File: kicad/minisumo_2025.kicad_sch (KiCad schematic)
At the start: 5 parts

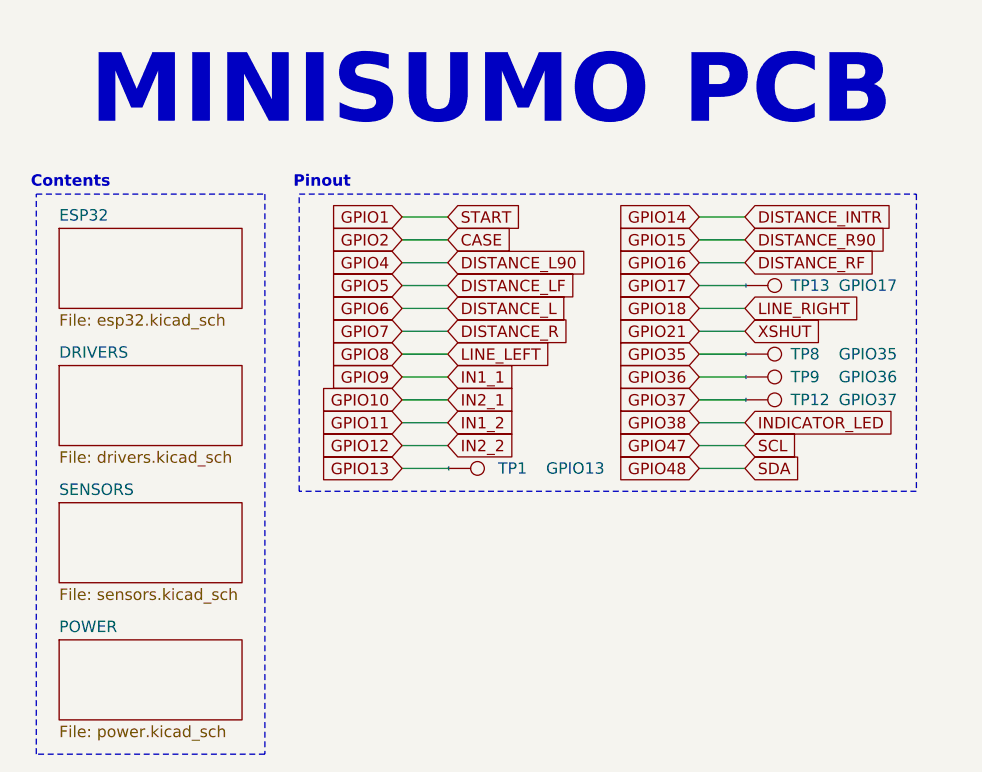
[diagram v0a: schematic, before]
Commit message: 2026 version
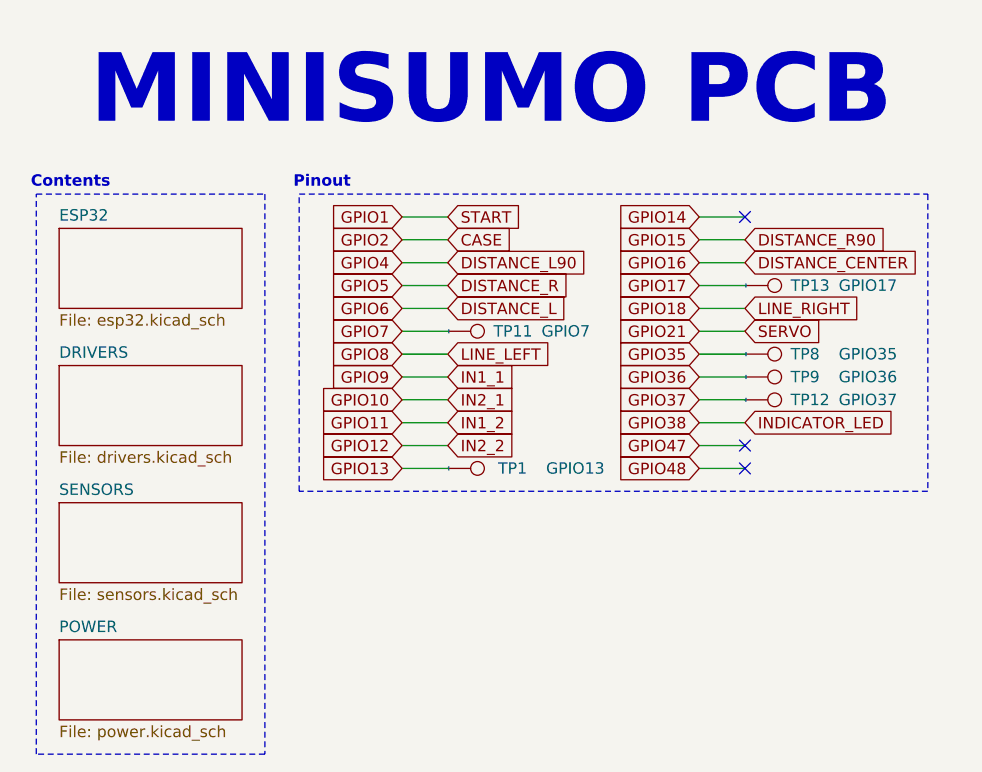
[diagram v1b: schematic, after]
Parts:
- added TP11: GPIO7, TestPoint:TestPoint_Pad_1.5x1.5mm, symbol Connector:TestPoint
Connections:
- new net GPIO7: TP11.1
- no-connect marks 0 -> 3
